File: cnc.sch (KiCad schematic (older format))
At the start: 22 parts, among them J1 Micro_SD_Card_Det, J16 Screw_Terminal_01x02, J2 Conn_01x02_Male, J3 Conn_01x02_Male, U1 LM324, U2 ESP32-DEVKITC, U3 AOZ1282CI, U4 AZ1117-3.3

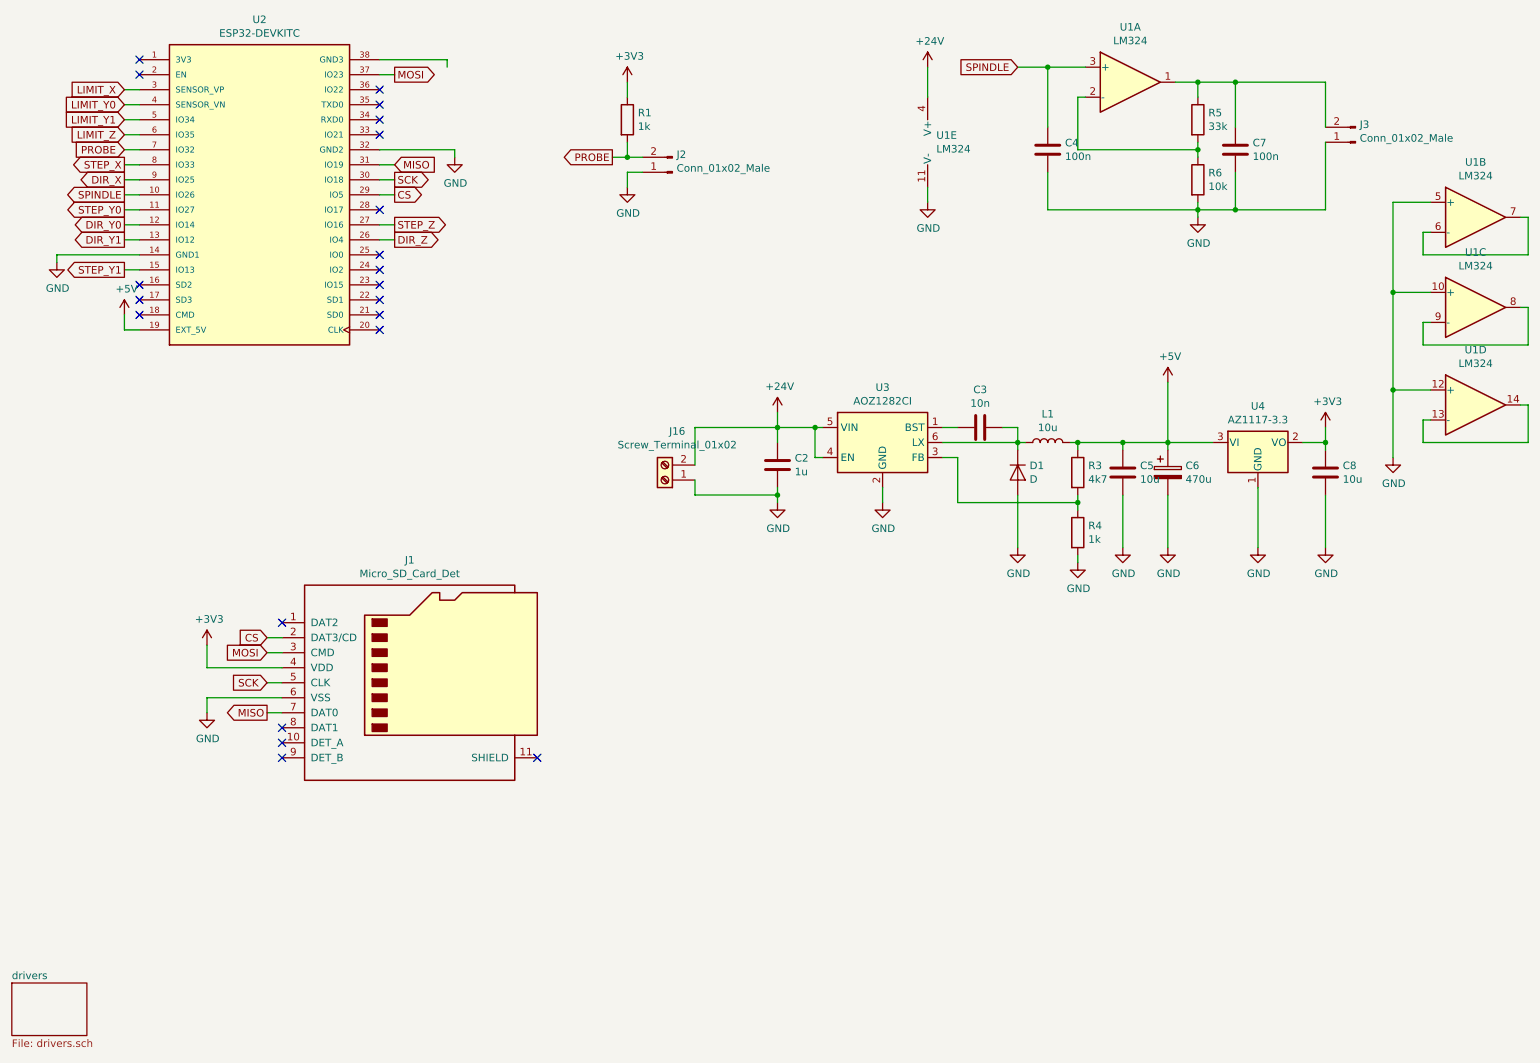
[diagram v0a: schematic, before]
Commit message: External drivers
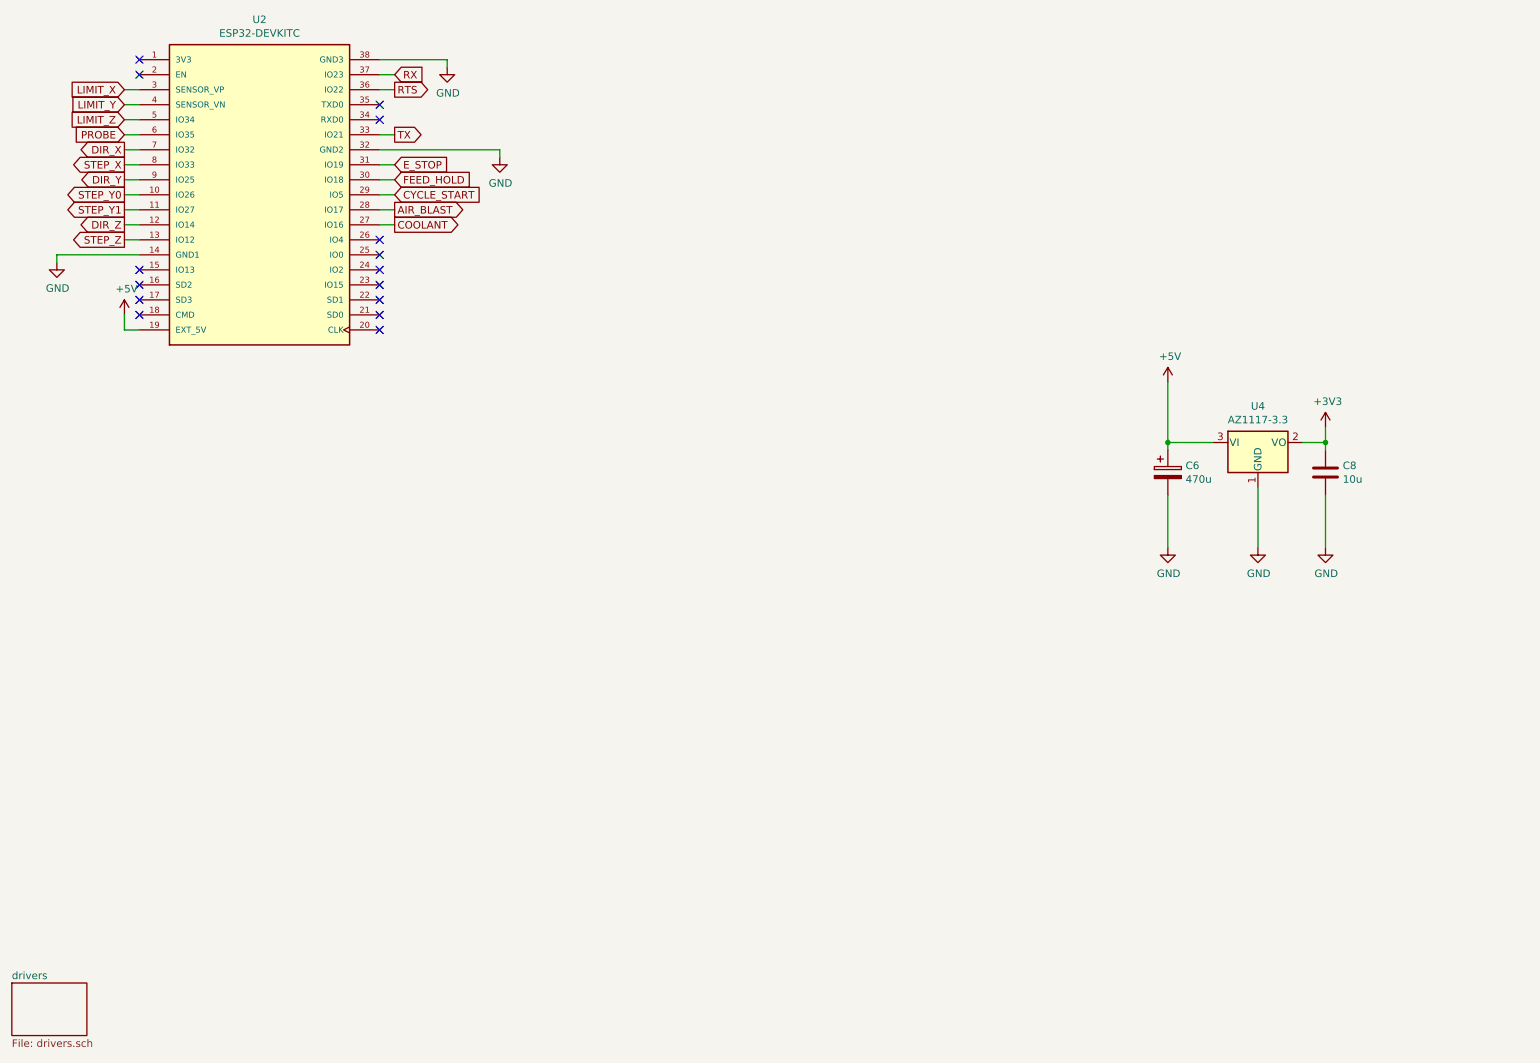
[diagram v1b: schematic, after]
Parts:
- removed C2: 1u, Capacitor_SMD:C_1206_3216Metric_Pad1.42x1.75mm_HandSolder, symbol Device:C
- removed C3: 10n, Capacitor_SMD:C_1206_3216Metric_Pad1.42x1.75mm_HandSolder, symbol Device:C
- removed C4, C7: 100n, Capacitor_SMD:C_1206_3216Metric_Pad1.42x1.75mm_HandSolder, symbol Device:C
- removed C5: 10u, Capacitor_SMD:C_1206_3216Metric_Pad1.42x1.75mm_HandSolder, symbol Device:C
- removed D1: D, Diode_SMD:D_SMA_Handsoldering, symbol Device:D
- removed J1: Micro_SD_Card_Det, Connector_Card:microSD_HC_Hirose_DM3D-SF, symbol Connector:Micro_SD_Card_Det
- removed J16: Screw_Terminal_01x02, TerminalBlock_MetzConnect:TerminalBlock_MetzConnect_Type011_RT05502HBWC_1x02_P5.00mm_Horizontal, symbol Connector:Screw_Terminal_01x02
- removed J2, J3: Conn_01x02_Male, Connector_PinHeader_2.54mm:PinHeader_1x02_P2.54mm_Vertical, symbol Connector:Conn_01x02_Male
- removed L1: 10u, Inductor_SMD:L_Bourns-SRN4018, symbol Device:L
- removed R1, R4: 1k, Resistor_SMD:R_1206_3216Metric_Pad1.42x1.75mm_HandSolder, symbol Device:R
- removed R3: 4k7, Resistor_SMD:R_1206_3216Metric_Pad1.42x1.75mm_HandSolder, symbol Device:R
- removed R5: 33k, Resistor_SMD:R_1206_3216Metric_Pad1.42x1.75mm_HandSolder, symbol Device:R
- removed R6: 10k, Resistor_SMD:R_1206_3216Metric_Pad1.42x1.75mm_HandSolder, symbol Device:R
- removed U1: LM324, Package_SO:SOIC-14_3.9x8.7mm_P1.27mm, symbol Amplifier_Operational:LM324
- removed U3: AOZ1282CI, Package_TO_SOT_SMD:SOT-23-6, symbol Regulator_Switching:AOZ1282CI
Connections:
- net DIR_Y0 is gone; now on net DIR_Z: U2.12 (IO14)
- net DIR_Y1 is gone; now on net STEP_Z: U2.13 (IO12)
- net LIMIT_Y1 is gone; now on net LIMIT_Z: U2.5 (IO34)
- net SPINDLE is gone; now on net STEP_Y0: U2.10 (IO26)
- net DIR_X: now also U2.7 (IO32); no longer U2.9 (IO25)
- net DIR_Z: no longer U2.26 (IO4)
- net GND: now also U2.38 (GND3)
- net LIMIT_Z: no longer U2.6 (IO35)
- net PROBE: now also U2.6 (IO35); no longer U2.7 (IO32)
- net STEP_Y0: no longer U2.11 (IO27)
- net STEP_Y1: now also U2.11 (IO27); no longer U2.15 (IO13)
- net STEP_Z: no longer U2.27 (IO16)
- net AIR_BLAST: now reaches U2.28 (IO17)
- net TX: now reaches U2.33 (IO21)
- net RTS: now reaches U2.36 (IO22)
- net CS renamed CYCLE_START
- net LIMIT_Y0 renamed LIMIT_Y
- net MISO renamed E_STOP
- net MOSI renamed RX
- net SCK renamed FEED_HOLD
- new net COOLANT: U2.27 (IO16)
- new net DIR_Y: U2.9 (IO25)
- no-connect marks 21 -> 15

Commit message: Fixes
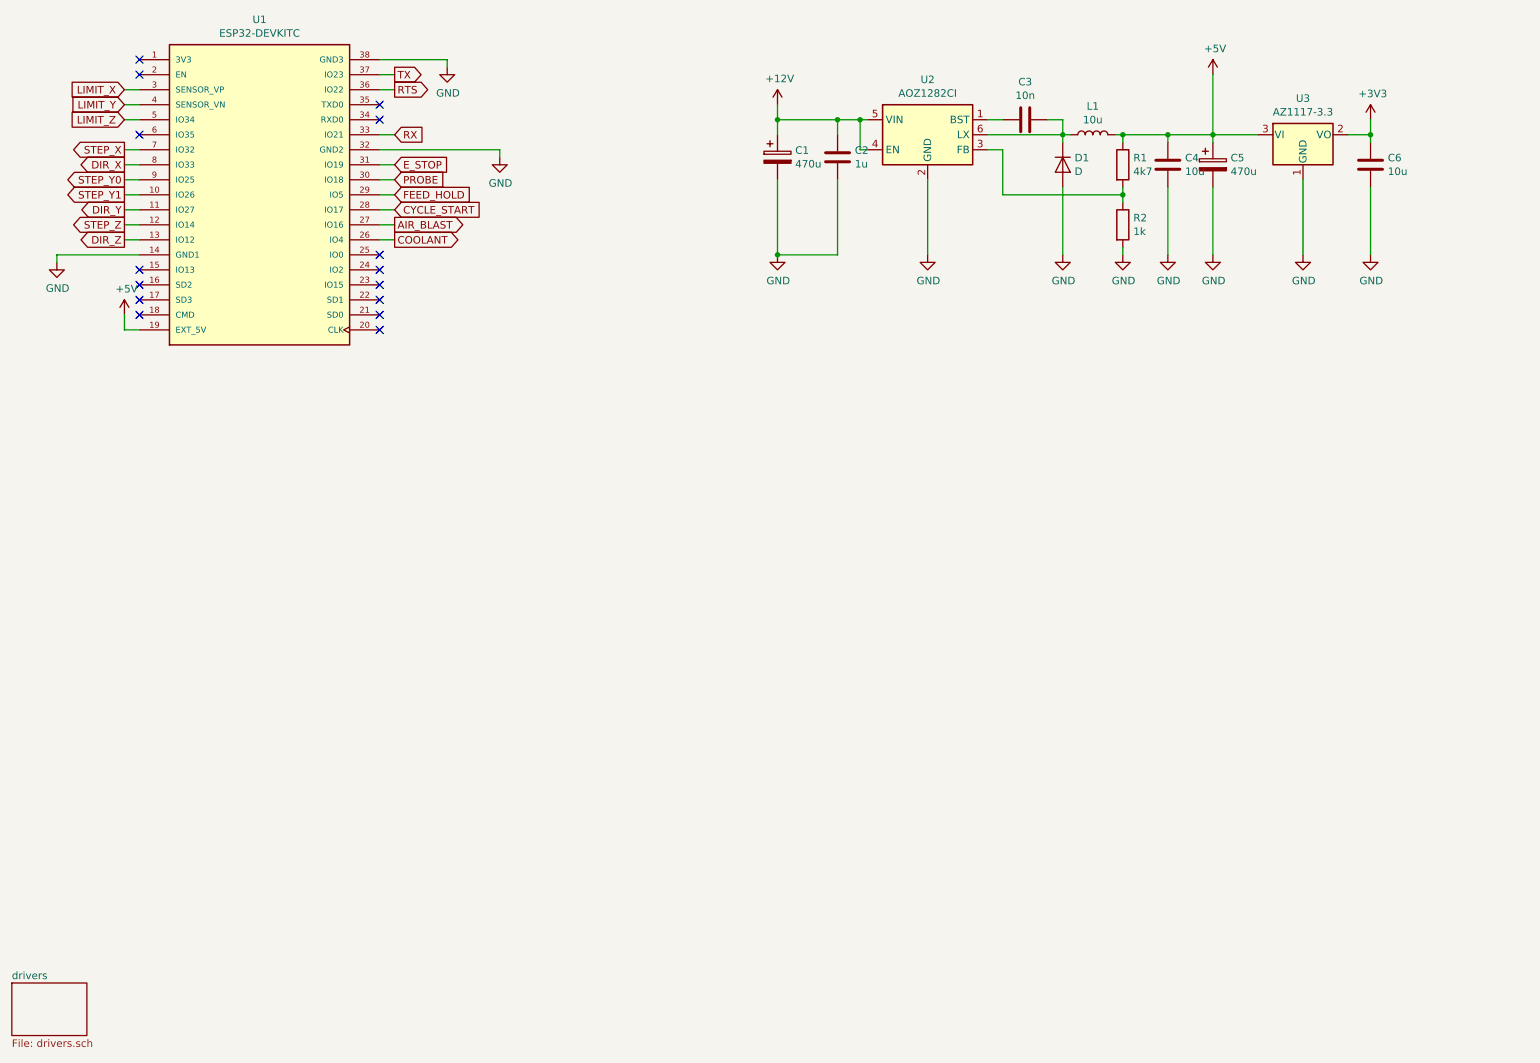
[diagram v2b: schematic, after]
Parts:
- removed C6: 470u, Capacitor_SMD:CP_Elec_8x10, symbol Device:CP
- removed C8: 10u, Capacitor_SMD:C_1206_3216Metric_Pad1.42x1.75mm_HandSolder, symbol Device:C
- removed U4: AZ1117-3.3, Package_TO_SOT_SMD:SOT-223-3_TabPin2, symbol Regulator_Linear:AZ1117-3.3
- added C1, C5: 470u, Capacitor_SMD:CP_Elec_8x10, symbol Device:CP
- added C2: 1u, Capacitor_SMD:C_1206_3216Metric_Pad1.42x1.75mm_HandSolder, symbol Device:C
- added C3: 10n, Capacitor_SMD:C_1206_3216Metric_Pad1.42x1.75mm_HandSolder, symbol Device:C
- added C4, C6: 10u, Capacitor_SMD:C_1206_3216Metric_Pad1.42x1.75mm_HandSolder, symbol Device:C
- added D1: D, Diode_SMD:D_SMA_Handsoldering, symbol Device:D
- added L1: 10u, Inductor_SMD:L_Bourns-SRN4018, symbol Device:L
- added R1: 4k7, Resistor_SMD:R_1206_3216Metric_Pad1.42x1.75mm_HandSolder, symbol Device:R
- added R2: 1k, Resistor_SMD:R_1206_3216Metric_Pad1.42x1.75mm_HandSolder, symbol Device:R
- added U2: AOZ1282CI, Package_TO_SOT_SMD:SOT-23-6, symbol Regulator_Switching:AOZ1282CI
- added U3: AZ1117-3.3, Package_TO_SOT_SMD:SOT-223-3_TabPin2, symbol Regulator_Linear:AZ1117-3.3
- renumbered U2 to U1
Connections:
- net +3V3: now also C6.1, U3.2 (VO)
- net +5V: now also C4.1, C5.1, L1.2, R1.1, U3.3 (VI)
- net AIR_BLAST: now also U1.27 (IO16); no longer U1.28 (IO17)
- net COOLANT: now also U1.26 (IO4); no longer U1.27 (IO16)
- net CYCLE_START: now also U1.28 (IO17); no longer U1.29 (IO5)
- net DIR_X: now also U1.8 (IO33); no longer U1.7 (IO32)
- net DIR_Y: now also U1.11 (IO27); no longer U1.9 (IO25)
- net DIR_Z: now also U1.13 (IO12); no longer U1.12 (IO14)
- net FEED_HOLD: now also U1.29 (IO5); no longer U1.30 (IO18)
- net GND: now also C1.2, C2.2, C4.2, C5.2, C6.2, D1.2 (A), R2.2, U2.2 (GND), U3.1 (GND)
- net PROBE: now also U1.30 (IO18); no longer U1.6 (IO35)
- net RX: now also U1.33 (IO21); no longer U1.37 (IO23)
- net STEP_X: now also U1.7 (IO32); no longer U1.8 (IO33)
- net STEP_Y0: now also U1.9 (IO25); no longer U1.10 (IO26)
- net STEP_Y1: now also U1.10 (IO26); no longer U1.11 (IO27)
- net STEP_Z: now also U1.12 (IO14); no longer U1.13 (IO12)
- net TX: now also U1.37 (IO23); no longer U1.33 (IO21)
- new net: R1.2, R2.1, U2.3 (FB)
- new net: C3.2, D1.1 (K), L1.1, U2.6 (LX)
- new net: C3.1, U2.1 (BST)
- new net +12V: C1.1, C2.1, U2.4 (EN), U2.5 (VIN)
